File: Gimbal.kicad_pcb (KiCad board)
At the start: 2 copper layers, 68.6 x 63.5 mm, 43 parts, among them J1 Conn_01x03, J2 USB_C_Receptacle_USB2.0, J3 0022232041, J4 0022232041, J5 0022232041, J6 Conn_01x02, Q1 Q_NPN_BCE, Q2 Q_NPN_BCE, SW1 SW_Push, U1 ESP32-S2-SOLO, U2 BMI088, U3 CP2102N-Axx-xQFN28, U4 TLV70433DBVT, U5 DRV8846RGET, U6 DRV8846RGET

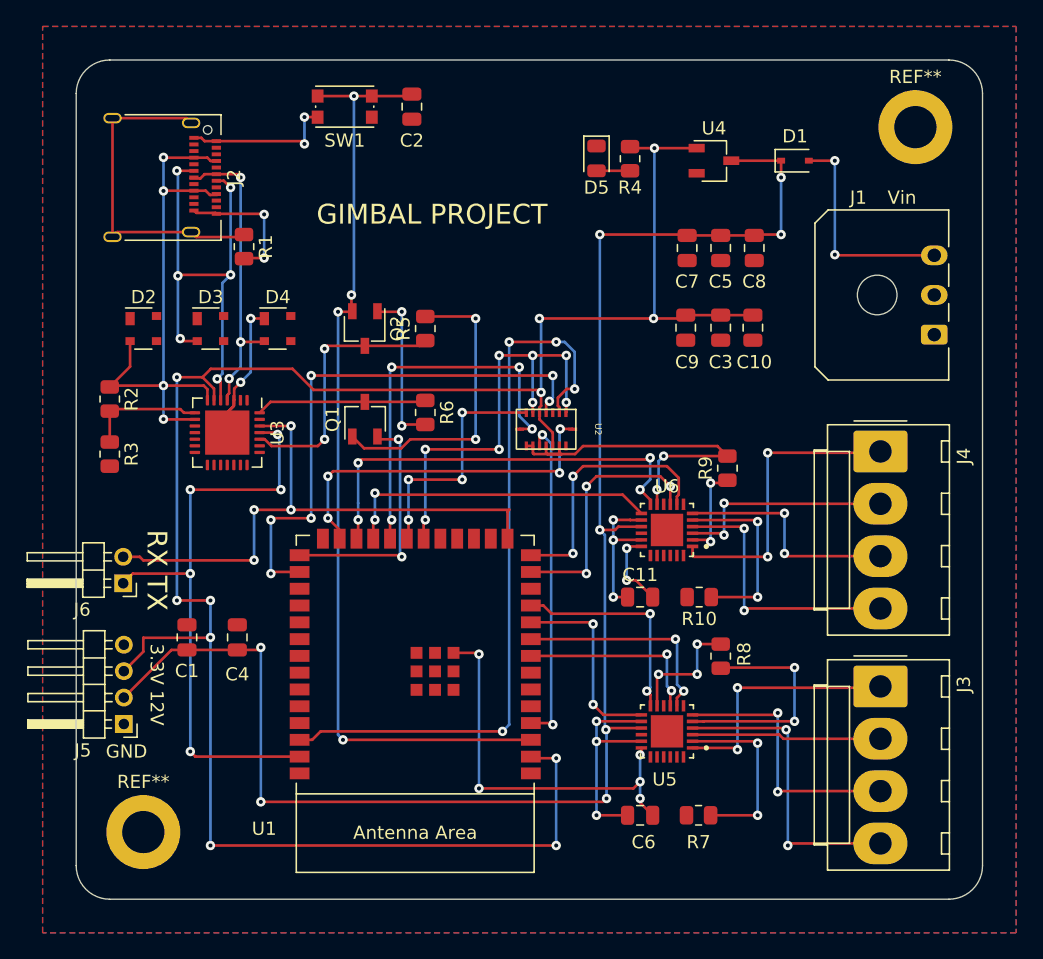
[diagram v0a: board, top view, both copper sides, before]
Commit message: started new layout
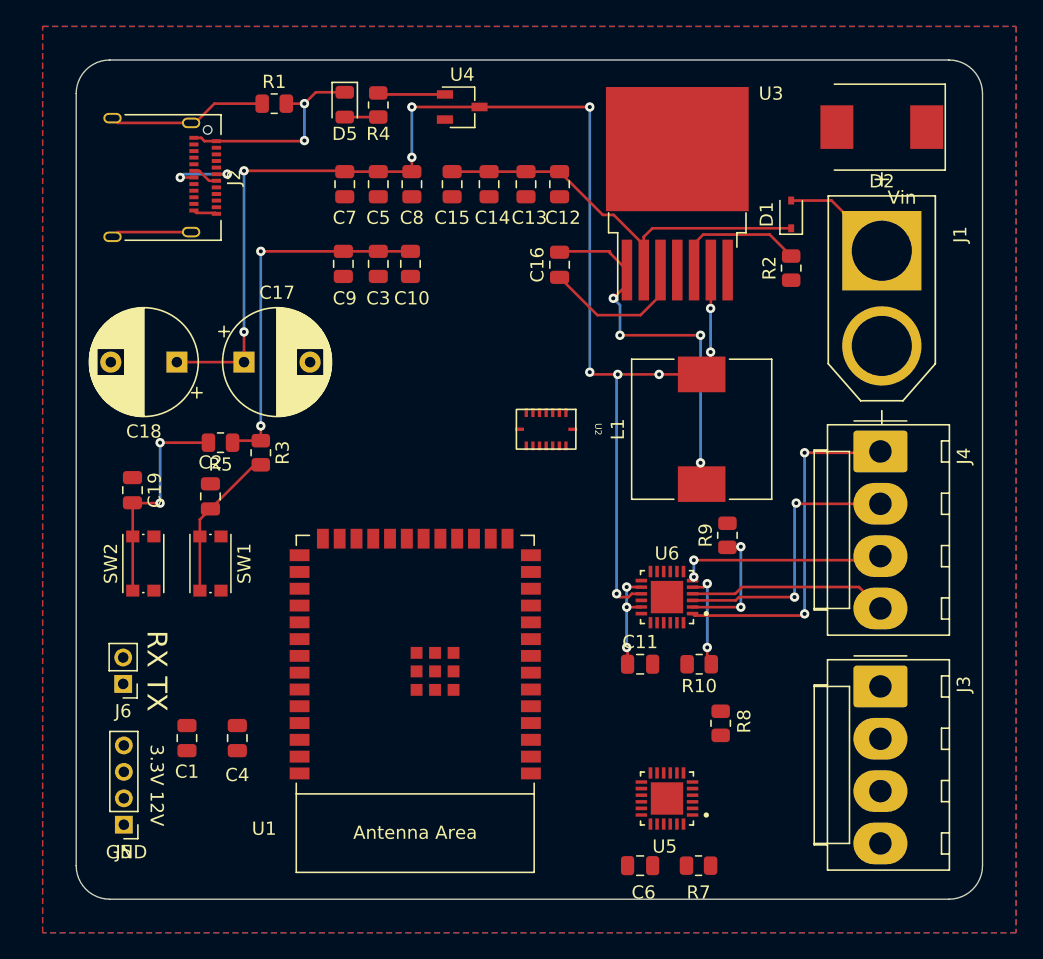
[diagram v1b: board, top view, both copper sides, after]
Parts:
- removed D3, D4: DIODE, Package_TO_SOT_SMD:SOT-143
- removed Q1, Q2: Q_NPN_BCE, Package_TO_SOT_SMD:TSOT-23
- removed R6: 10k, Resistor_SMD:R_0805_2012Metric
- removed REF** (x2): MountingHole_3.2mm_M3_DIN965_Pad, MountingHole:MountingHole_3.2mm_M3_DIN965_Pad
- added C12: 15uF, Capacitor_SMD:C_0805_2012Metric, F.Cu at (150.9, 70.4)
- added C13: 15uF, Capacitor_SMD:C_0805_2012Metric, F.Cu at (148.3, 70.4)
- added C14: 15uF, Capacitor_SMD:C_0805_2012Metric, F.Cu at (145.5, 70.4)
- added C15: 0.47 uF, Capacitor_SMD:C_0805_2012Metric, F.Cu at (142.7, 70.4)
- added C16: .01uF, Capacitor_SMD:C_0805_2012Metric, F.Cu at (150.9, 76.5)
- added C17: 180uF, Capacitor_THT:CP_Radial_D8.0mm_P5.00mm, F.Cu at (127.0, 83.8)
- added C18: 180uF, Capacitor_THT:CP_Radial_D8.0mm_P5.00mm, F.Cu at (121.9, 83.8)
- added C19: 0.1uF, Capacitor_SMD:C_0805_2012Metric, F.Cu at (118.6, 93.5)
- added L1: 22uH, Inductor_SMD:L_10.4x10.4_H4.8, F.Cu at (161.6, 88.9)
- added SW2: SW_Push, Button_Switch_SMD:SW_Push_1P1T_NO_CK_KMR2, F.Cu at (119.4, 99.1)
- D2: footprint Package_TO_SOT_SMD:SOT-143 -> Diode_SMD:D_SMC
- J1: value Conn_01x03 -> XT60-M; footprint Connector_Molex:Molex_Micro-Fit_3.0_43650-0300_1x03_P3.00mm_Horizontal -> GIMBAL:AMASS_XT60-M
- J5: footprint Connector_PinHeader_2.00mm:PinHeader_1x04_P2.00mm_Horizontal -> Connector_PinHeader_2.00mm:PinHeader_1x04_P2.00mm_Vertical
- J6: footprint Connector_PinHeader_2.00mm:PinHeader_1x02_P2.00mm_Horizontal -> Connector_PinHeader_2.00mm:PinHeader_1x02_P2.00mm_Vertical
- R2: value 22.1k -> 5.6k
- R3: value 47.5k -> 10k
- U3: value CP2102N-Axx-xQFN28 -> LM2679SX-12; footprint Package_DFN_QFN:QFN-28-1EP_5x5mm_P0.5mm_EP3.35x3.35mm -> Package_TO_SOT_SMD:TO-263-7_TabPin8
- moved D2 57.9 mm to (175.3, 66.0), turned to 180 degrees
- moved R2 52.5 mm to (168.4, 76.7), turned to 90 degrees
- moved U3 38.6 mm to (159.8, 71.1), turned to 90 degrees
- moved SW1 36.0 mm to (124.5, 99.1), turned to 90 degrees
- moved C2 33.2 mm to (124.5, 94.0), turned to -90 degrees
- moved C3 26.4 mm to (137.2, 76.4)
- moved C5 26.4 mm to (137.2, 70.4)
- moved C8 26.4 mm to (139.7, 70.4)
- moved C9 26.4 mm to (134.5, 76.4)
- moved C10 26.4 mm to (139.6, 76.4)
- moved C7 26.4 mm to (134.6, 70.4)
- moved R4 19.5 mm to (137.2, 64.4)
- moved U4 19.5 mm to (143.5, 64.5)
- moved D5 19.5 mm to (134.6, 64.3)
- moved R5 17.7 mm to (125.2, 89.9), turned to 180 degrees
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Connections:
- D1 pad 1: +12V -> +BATT
- D2 pad 2: /VBUS -> Net-(C16-Pad2)
- J2 pad A4: /VBUS -> unconnected-(J2-PadA4)
- J2 pad A6: Net-(D4-Pad2) -> /D+
- J2 pad A7: Net-(D3-Pad2) -> /D-
- J2 pad A9: /VBUS -> unconnected-(J2-PadA4)
- J2 pad B4: /VBUS -> unconnected-(J2-PadA4)
- J2 pad B6: Net-(D4-Pad2) -> /D+
- J2 pad B7: Net-(D3-Pad2) -> /D-
- J2 pad B9: /VBUS -> unconnected-(J2-PadA4)
- R2 pad 1: /VBUS -> GND
- R3 pad 1: Net-(R2-Pad2) -> +3V3
- R3 pad 2: GND -> /EN
- R5 pad 1: /!RTS -> +3V3
- R5 pad 2: Net-(Q1-Pad1) -> /GPIO0
- U1 pad 10: /Motor1Dir -> unconnected-(U1-Pad10)
- U1 pad 11: /Motor1Step -> unconnected-(U1-Pad11)
- U1 pad 12: unconnected-(U1-Pad12) -> /Motor1Step
- U1 pad 13: /Motor2M1 -> /D-
- U1 pad 14: /Motor2M0 -> /D+
- U1 pad 17: unconnected-(U1-Pad17) -> /Motor2M1
- U1 pad 18: unconnected-(U1-Pad18) -> /Motor2M0
- U1 pad 19: unconnected-(U1-Pad19) -> /Motor2Dir
- U1 pad 23: /Motor2Dir -> unconnected-(U1-Pad23)
- U1 pad 24: /Motor2Step -> unconnected-(U1-Pad24)
- U1 pad 5: unconnected-(U1-Pad5) -> /Motor1M1
- U1 pad 6: unconnected-(U1-Pad6) -> /Motor1M0
- U1 pad 7: unconnected-(U1-Pad7) -> /Motor1Dir
- U1 pad 8: /Motor1M1 -> /Motor2Step
- U1 pad 9: /Motor1M0 -> unconnected-(U1-Pad9)
- U3 pad 1: unconnected-(U3-Pad1) -> Net-(C16-Pad2)
- U3 pad 2: unconnected-(U3-Pad2) -> +BATT
- U3 pad 3: GND -> /BUCKCB
- U3 pad 4: Net-(D4-Pad2) -> GND
- U3 pad 5: Net-(D3-Pad2) -> Net-(R2-Pad2)
- U3 pad 6: +3V3 -> +12V
- U3 pad 7: /VBUS -> unconnected-(U3-Pad7)
- U3 pad 8: Net-(R2-Pad2) -> (no net)
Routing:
- net +3V3: track 156.0 -> 32.9 mm, vias 11 -> 2
- net GND: track 105.8 -> 17.9 mm, vias 18 -> 2
- net /EN: track 72.0 -> 11.7 mm, vias 4 -> 0
- net /ESPIO2: track 56.1 -> 0.00 mm, vias 4 -> 0
- net /ESPTX: track 46.2 -> 0.00 mm, vias 5 -> 0
- net /ESPRX: track 44.1 -> 0.00 mm, vias 4 -> 0
- net /VBUS: track 43.0 -> 0.00 mm, vias 4 -> 0
- net /ESPIO35: track 41.5 -> 0.00 mm, vias 6 -> 0
- net Net-(D3-Pad2): track 37.4 -> 0.00 mm, vias 6 -> 0
- net /SPI_MISO: track 33.3 -> 0.00 mm, vias 8 -> 0
- net +BATT: track 0.00 -> 32.6 mm
- net /Motor2Step: track 32.2 -> 0.00 mm, vias 4 -> 0
- net /SPI_CLK: track 28.8 -> 0.00 mm, vias 4 -> 0
- net Net-(C16-Pad2): track 0.00 -> 28.8 mm, vias 0 -> 4
- net /ESPIO34: track 27.1 -> 0.00 mm, vias 4 -> 0
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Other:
- board text removed: "GIMBAL PROJECT"
